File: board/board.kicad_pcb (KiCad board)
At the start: 2 copper layers, 21 x 13 mm, 1 part

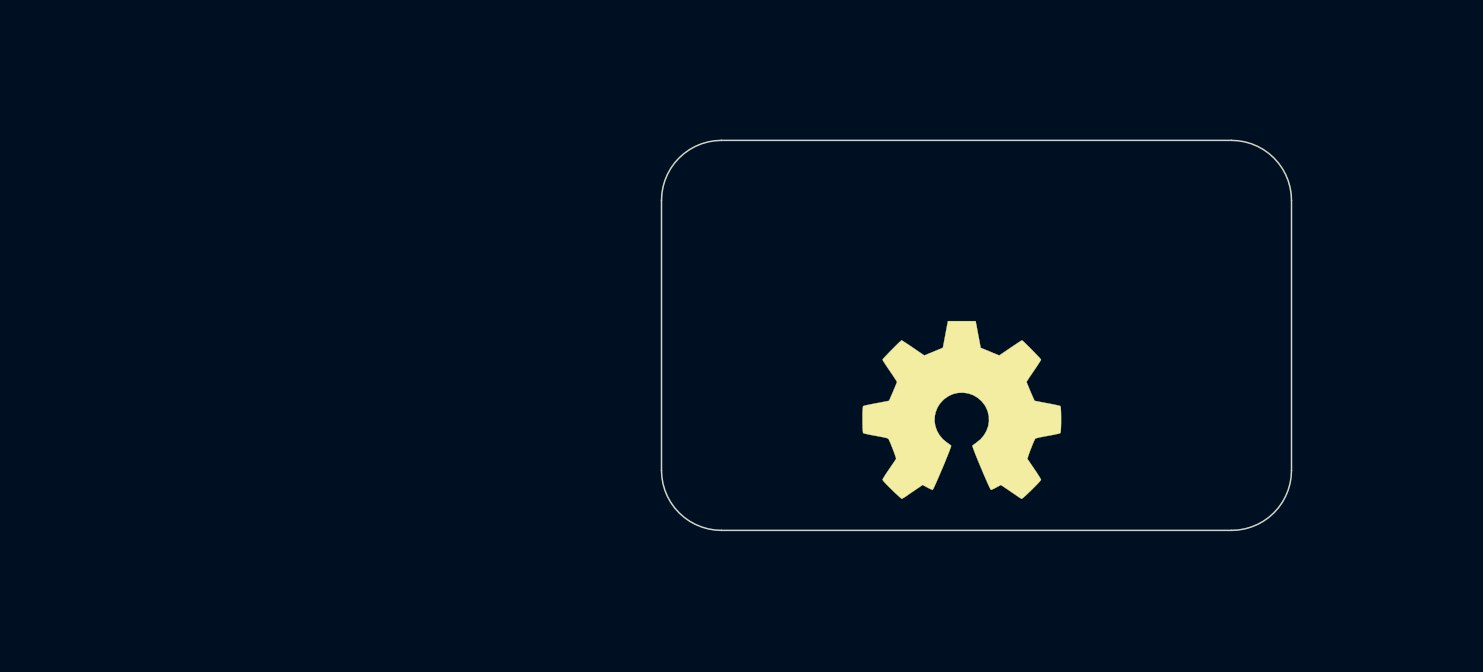
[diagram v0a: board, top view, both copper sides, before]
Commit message: initial
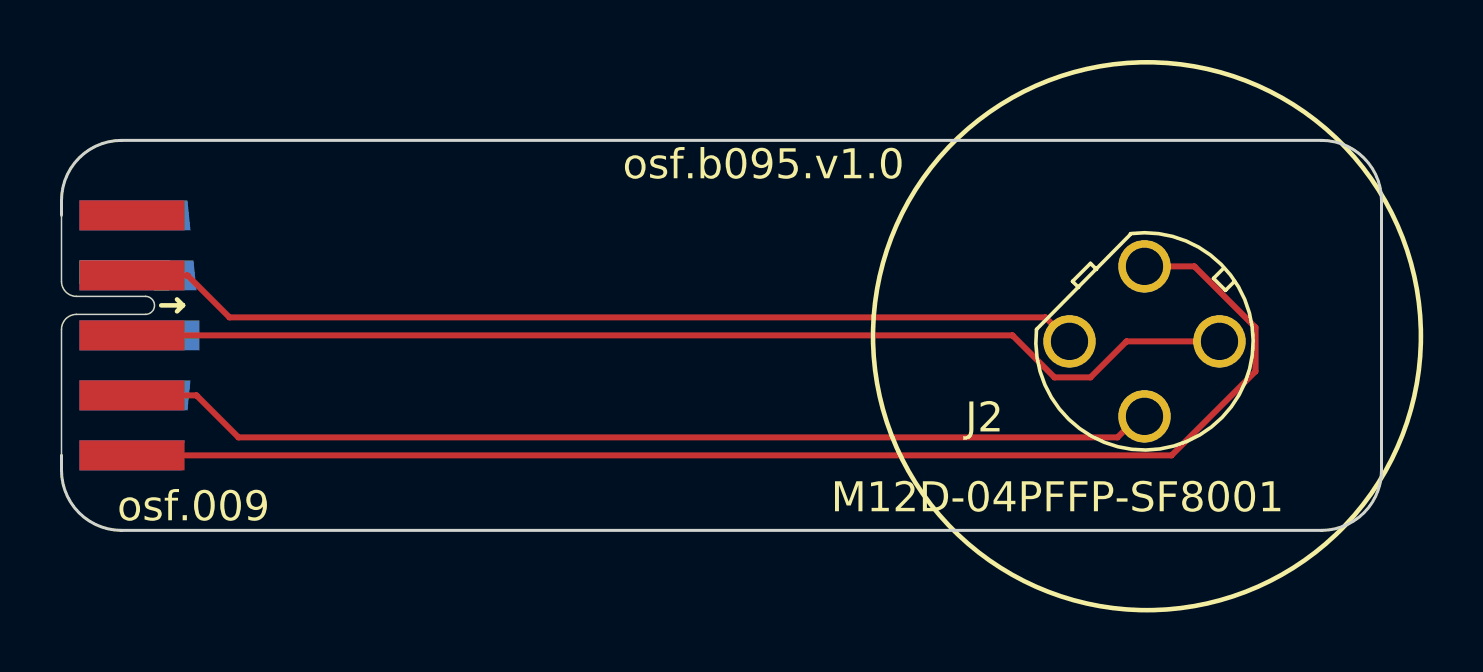
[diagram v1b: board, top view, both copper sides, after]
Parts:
- removed LOGO1: Logo_Open_Hardware_Small, Symbol:OSHW-Symbol_6.7x6mm_SilkScreen
- added J1: 009_1000BASE-T, on_edge:on_edge_2x05_device, F.Cu at (120.0, 96.5)
- added J2: M12D-04PFFP-SF8001, b095:M12D, F.Cu at (156.1, 96.7)
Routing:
- net /magnetics/RX-: track 0.00 -> 44.6 mm
- net /magnetics/TX-: track 0.00 -> 37.3 mm
- net /magnetics/RX+: track 0.00 -> 34.6 mm
- net /magnetics/TX+: track 0.00 -> 32.2 mm
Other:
- board size 21 x 13 mm -> 44 x 13 mm
- board text added: "osf.009"
- board text added: "osf.b095.v1.0"
